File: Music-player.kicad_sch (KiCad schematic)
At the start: 101 parts, among them J1 USB_C_Receptacle_USB2.0_14P, J2 Screw_Terminal_01x04, J3 Screw_Terminal_01x02, J4 MSD-4-A, J5 SJ-43514, Q2 DMG2301L, SW1 RESET, SW2 PLAY/STOP, SW3 SKIP, SW4 EXIT, SW5 OPTIONS, SW6 EC11_L, SW7 POWER, U1 TVS1400DRV, U2 nRF5340-QKxx, U3 SPX3819M5-L-3-3, U5 MCP73831-2-OT, U6 TPA6132A2RTE, U8 PCM5102A, Y1 MU00525-32-768K, Y2 ECS-320-8-37B-CKY-TR

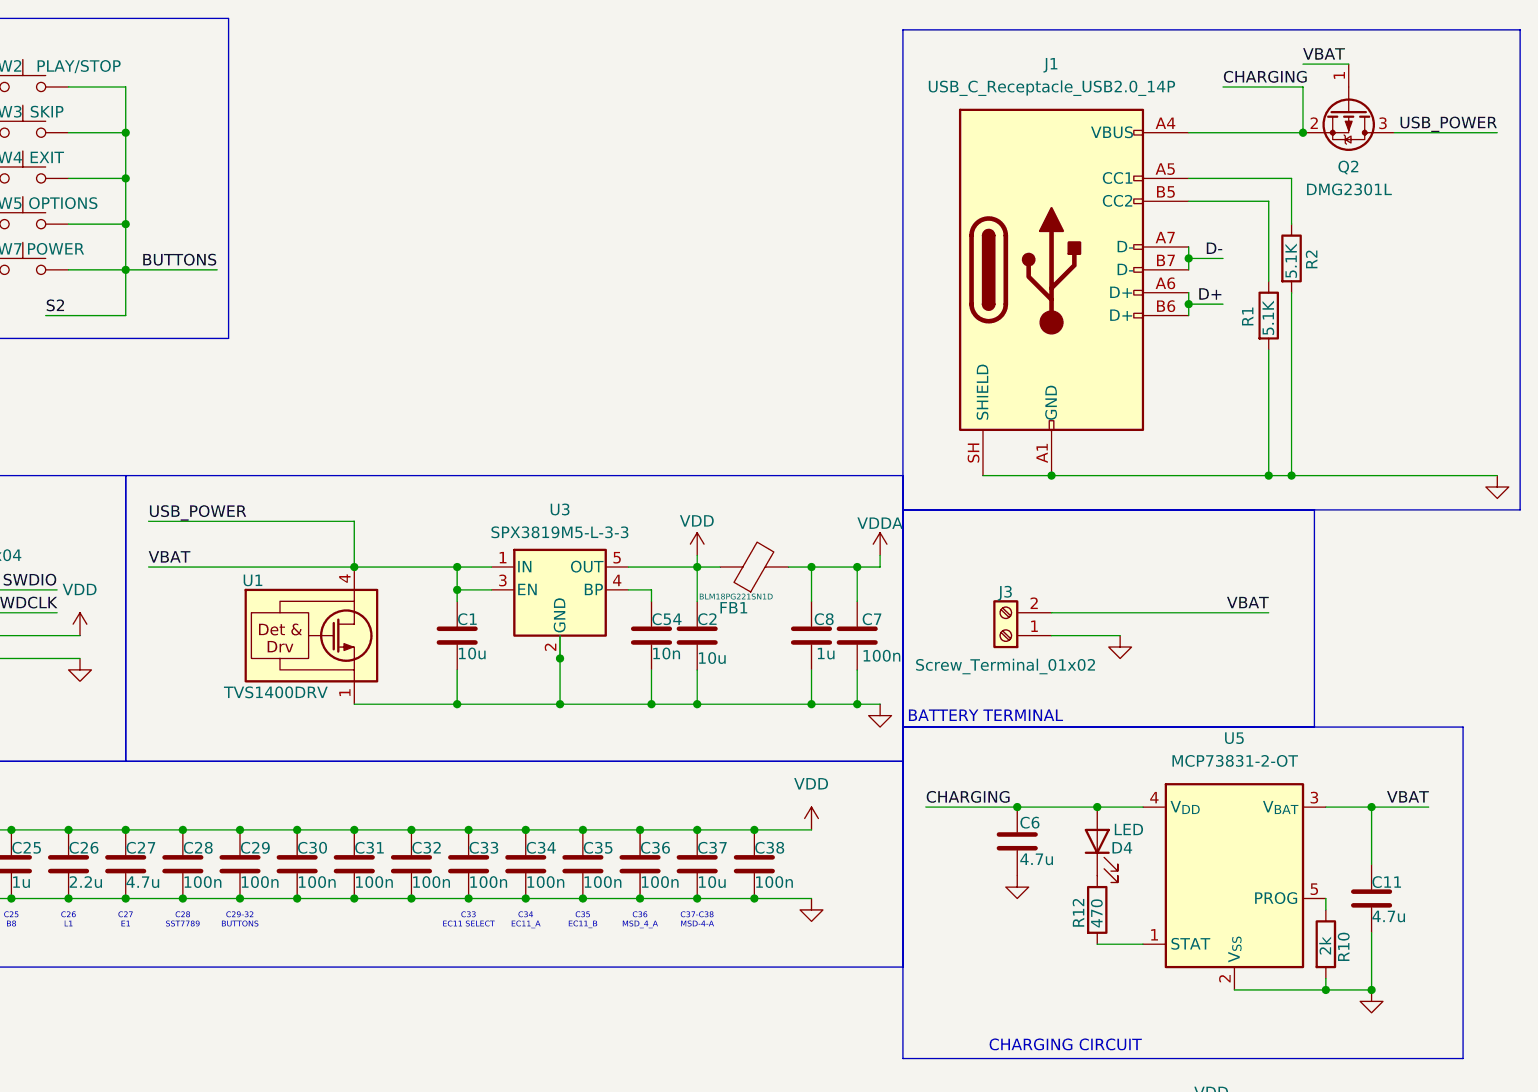
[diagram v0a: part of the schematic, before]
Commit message: Add files via upload
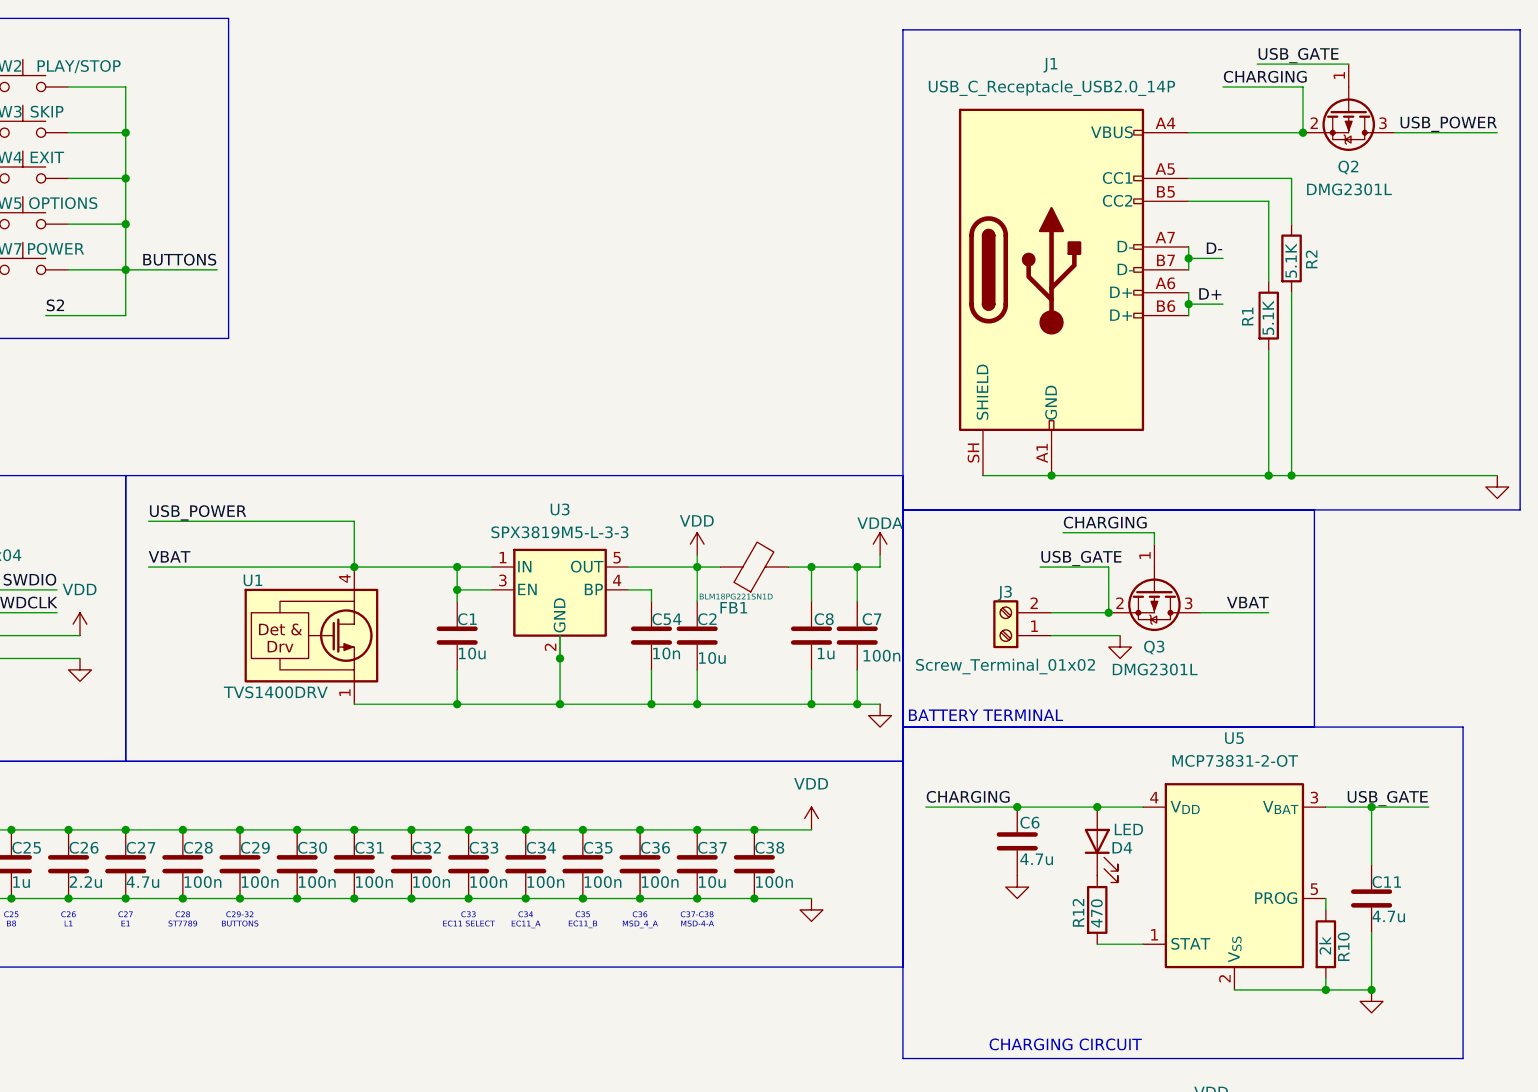
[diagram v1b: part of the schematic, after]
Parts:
- added Q3: DMG2301L, Package_TO_SOT_SMD:SOT-23, symbol Transistor_FET:DMG2301L
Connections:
- net CHARGING: now also Q3.1 (G)
- net USB_POWER: now also Q3.3 (D); no longer C11.1, J3.2 (Pin_2), Q2.1 (G), U5.3 (V_{BAT})
- new net USB_GATE: C11.1, J3.2 (Pin_2), Q2.1 (G), Q3.2 (S), U5.3 (V_{BAT})
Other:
- note added: "C28 ST7789"
- note removed: "C28 SST7789"
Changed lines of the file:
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@@
 		)
 	)
-	(text "C28\nSST7789\n"
+	(text "C28\nST7789\n"
 		(exclude_from_sim no)
 		(at 260.35 115.57 0)
@@
 	)
 	(junction
+		(at 363.22 81.28)
+		(diameter 0)
+		(color 0 0 0 0)
+	)
+	(junction
 		(at 335.28 91.44)
 		(diameter 0)
@@
 	(wire
 		(pts
+			(xy 363.22 81.28) (xy 363.22 76.2)
+		)
+		(stroke
+			(width 0)
+			(type default)
+		)
+	)
+	(wire
+		(pts
 			(xy 383.54 45.72) (xy 383.54 66.04)
 		)
@@
 	(wire
 		(pts
+			(xy 368.3 73.66) (xy 368.3 72.39)
+		)
+		(stroke
+			(width 0)
+			(type default)
+		)
+	)
+	(wire
+		(pts
 			(xy 254 43.18) (xy 264.16 43.18)
 		)
@@
 	(wire
 		(pts
-			(xy 356.87 81.28) (xy 381 81.28)
+			(xy 356.87 81.28) (xy 363.22 81.28)
 		)
 		(stroke
@@
 	(wire
 		(pts
+			(xy 373.38 81.28) (xy 381 81.28)
+		)
+		(stroke
+			(width 0)
+			(type default)
+		)
+	)
+	(wire
+		(pts
 			(xy 304.8 113.03) (xy 311.15 113.03)
 		)
@@
 	(wire
 		(pts
-			(xy 384.81 20.32) (xy 389.89 20.32)
+			(xy 379.73 20.32) (xy 389.89 20.32)
 		)
 		(stroke
@@
 	(wire
 		(pts
+			(xy 363.22 76.2) (xy 355.6 76.2)
+		)
+		(stroke
+			(width 0)
+			(type default)
+		)
+	)
+	(wire
+		(pts
 			(xy 254 43.18) (xy 254 48.26)
 		)
@@
 	(wire
 		(pts
+			(xy 368.3 72.39) (xy 358.14 72.39)
+		)
+		(stroke
+			(width 0)
+			(type default)
+		)
+	)
+	(wire
+		(pts
 			(xy 163.83 128.27) (xy 152.4 128.27)
 		)
@@
 		)
 	)
+	(label "USB_GATE"
+		(at 355.6 76.2 0)
+		(effects
+			(font
+				(size 1.27 1.27)
+			)
+			(justify left bottom)
+		)
+	)
 	(label "EC11_A"
 		(at 185.42 80.01 0)
@@
 		)
 	)
+	(label "CHARGING"
+		(at 358.14 72.39 0)
+		(effects
+			(font
+				(size 1.27 1.27)
+			)
+			(justify left bottom)
+		)
+	)
 	(label "SWDIO"
 		(at 77.47 77.47 0)
@@
 		)
 	)
-	(label "VBAT"
+	(label "USB_GATE"
 		(at 398.78 102.87 180)
 		(effects
@@
 		)
 	)
-	(label "VBAT"
-		(at 384.81 20.32 0)
+	(label "USB_GATE"
+		(at 379.73 20.32 0)
 		(effects
 			(font
@@
 					(unit 1)
 				)
+			)
+		)
+	)
+	(symbol
+		(lib_id "Transistor_FET:DMG2301L")
+		(at 368.3 78.74 270)
+		(unit 1)
+		(body_style 1)
+		(exclude_from_sim no)
+		(in_bom yes)
+		(on_board yes)
+		(in_pos_files yes)
+		(dnp no)
+		(fields_autoplaced yes)
+		(property "Reference" "Q3"
+			(at 368.3 85.09 90)
+			(show_name no)
+			(do_not_autoplace no)
+			(effects
+				(font
+					(size 1.27 1.27)
+				)
+			)
+		)
+		(property "Value" "DMG2301L"
+			(at 368.3 87.63 90)
+			(show_name no)
+			(do_not_autoplace no)
+			(effects
+				(font
+					(size 1.27 1.27)
+				)
+			)
+		)
+		(property "Footprint" "Package_TO_SOT_SMD:SOT-23"
+			(at 366.395 83.82 0)
+			(hide yes)
+			(show_name no)
+			(do_not_autoplace no)
+			(effects
+				(font
+					(size 1.27 1.27)
+					(italic yes)
+				)
+				(justify left)
+			)
+		)
+		(property "Datasheet" "https://www.diodes.com/assets/Datasheets/DMG2301L.pdf"
+			(at 364.49 83.82 0)
+			(hide yes)
+			(show_name no)
+			(do_not_autoplace no)
+			(effects
+				(font
+					(size 1.27 1.27)
+				)
+				(justify left)
+			)
+		)
+		(property "Description" "-3A Id, -20V Vds, P-Channel MOSFET, SOT-23"
+			(at 368.3 78.74 0)
+			(hide yes)
+			(show_name no)
+			(do_not_autoplace no)
+			(effects
+				(font
+					(size 1.27 1.27)
+				)
+			)
+		)
+		(pin "1"
+		)
+		(pin "3"
+		)
+		(pin "2"
+		)
+		(instances
+			(project "Music-player"
+				(path "/f98d3056-e9c6-4dc5-a080-338d8b2650d2"
+					(reference "Q3")
+					(unit 1)
+				)
